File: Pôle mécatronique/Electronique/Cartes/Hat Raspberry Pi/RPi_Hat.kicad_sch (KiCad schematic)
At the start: 30 parts, among them J1 Arrêt d'urgence, J2 RPi_GPIO, J3 Goupille, J4 Tension I2C, J5 I2C, U1 XBee, U2 MCP25625-x-SS, Y1 8MHz

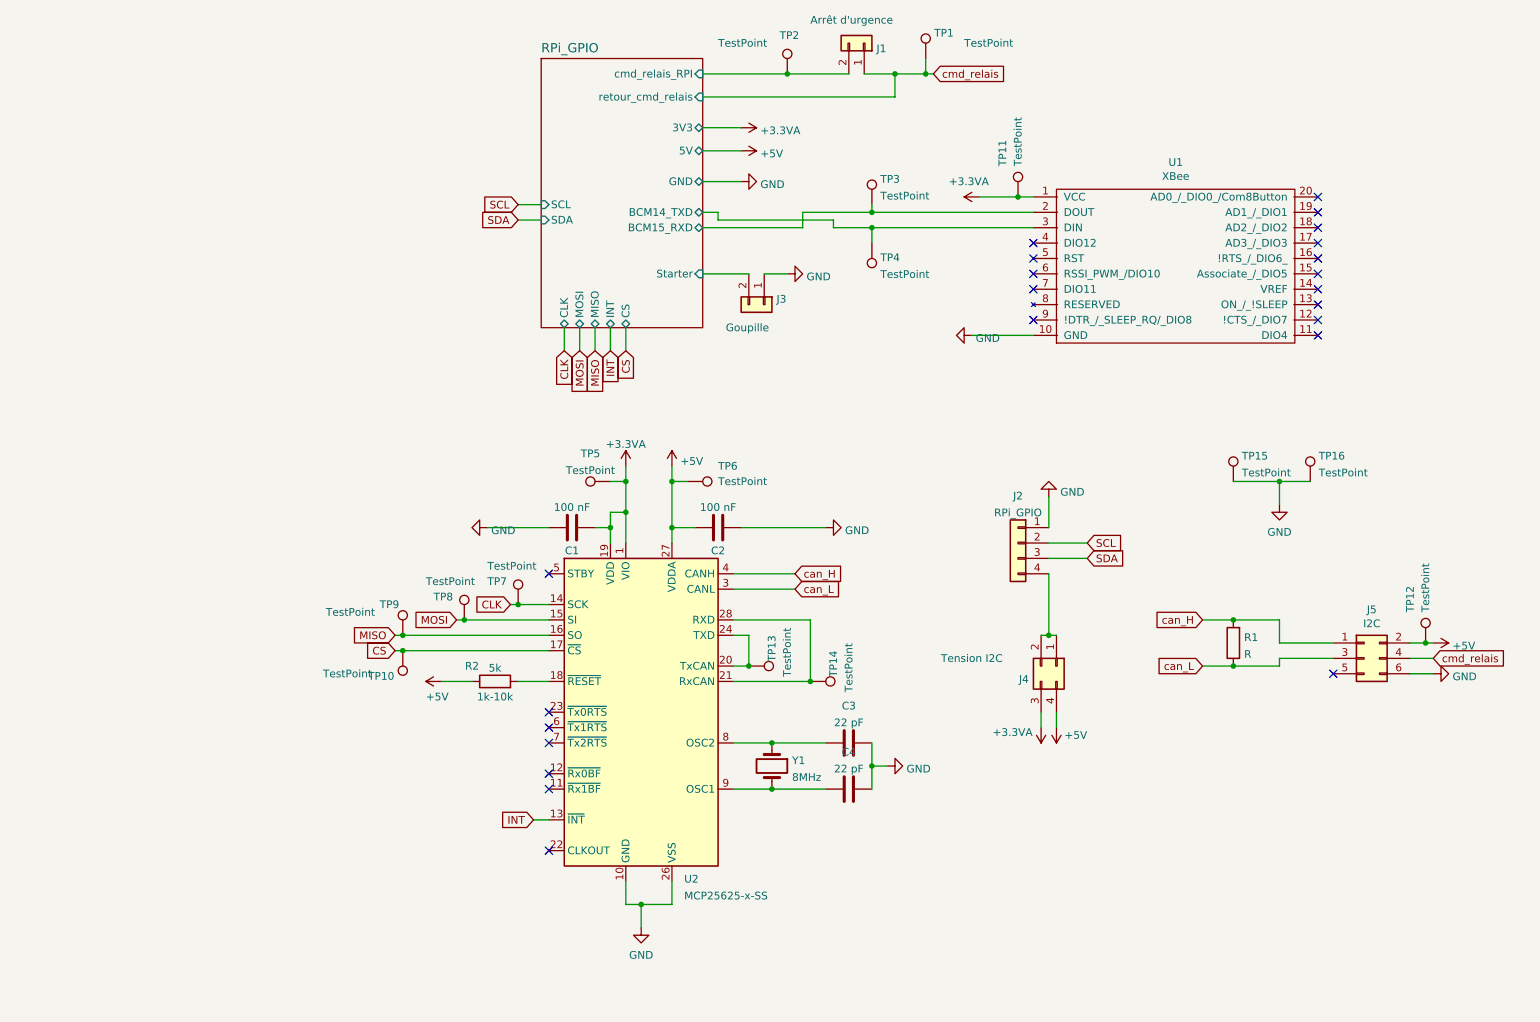
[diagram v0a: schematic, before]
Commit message: Up random
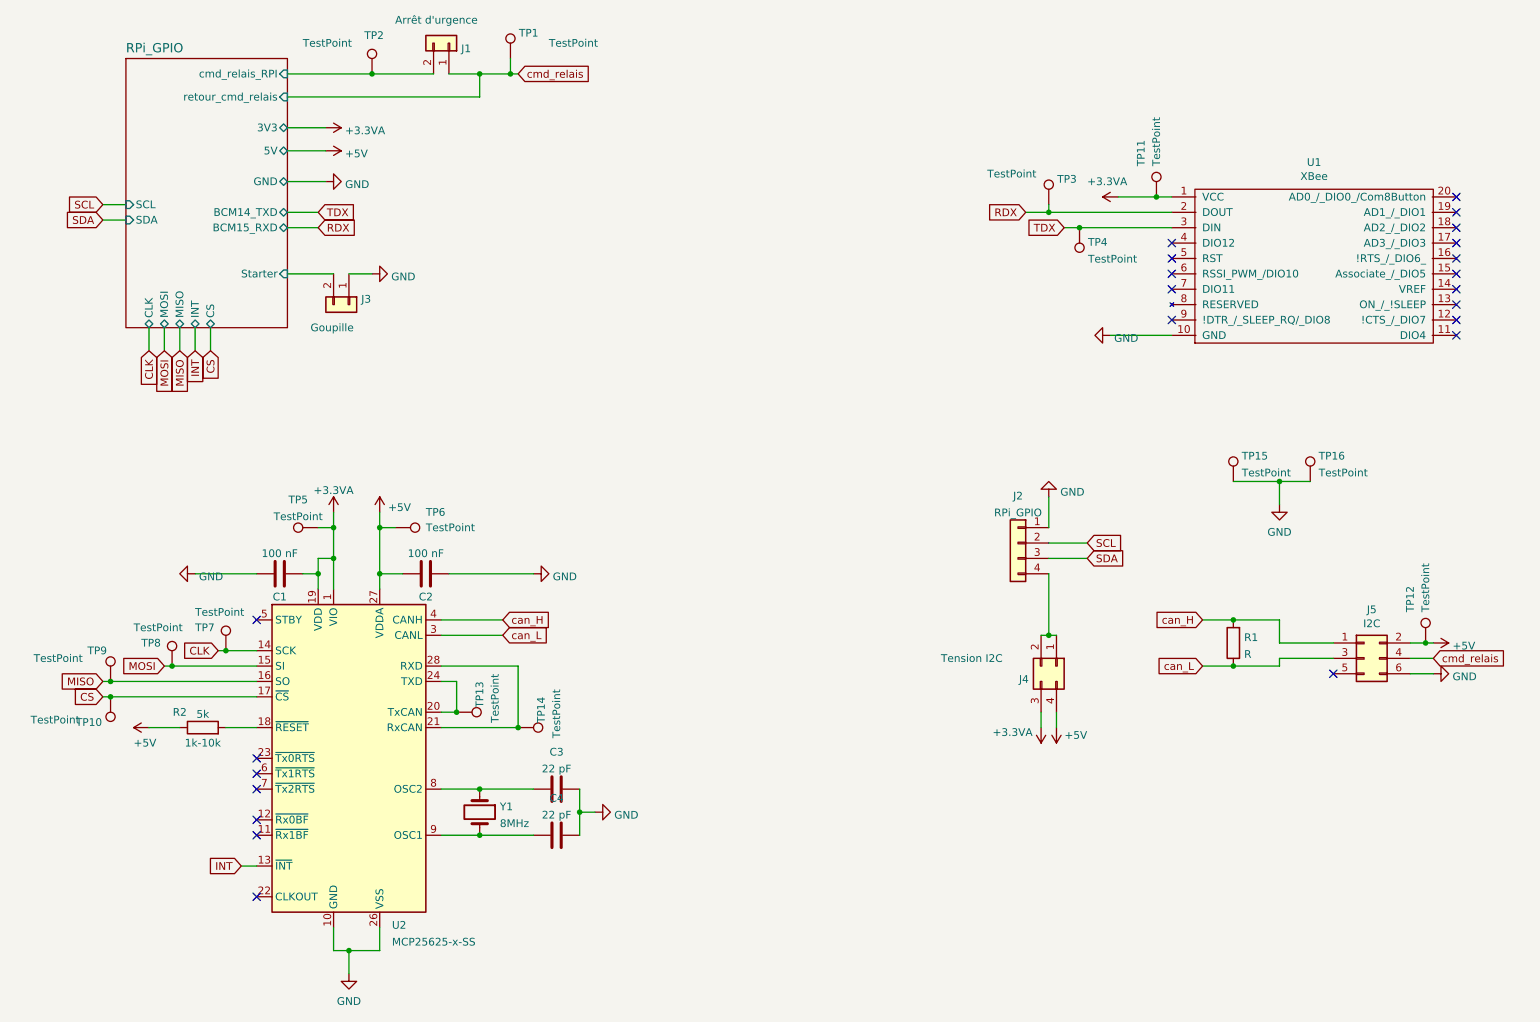
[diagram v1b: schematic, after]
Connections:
- net RPi_GPIO/BCM14_TXD renamed TDX
- net RPi_GPIO/BCM15_RXD renamed RDX
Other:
- moved on the sheet: C1, C2, C3, C4, J1, J3, R2, TP1, TP10, TP11, TP13, TP14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
